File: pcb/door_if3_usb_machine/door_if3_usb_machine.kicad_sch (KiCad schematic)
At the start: 75 parts, among them J1 Conn_01x08, J2 Conn_02x05_Odd_Even, J3 Conn_01x08, Q1 IRF7343, Q2 IRF7343, Q3 IRF7343, Q4 IRF7343, Q5 IRF7343, Q6 IRF7343, U1 Pico, U2 LTV-247, U4 LTV-247

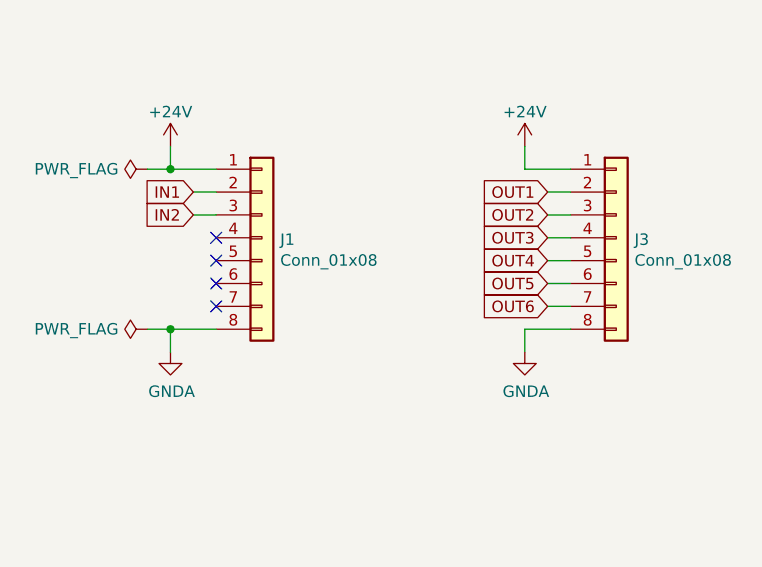
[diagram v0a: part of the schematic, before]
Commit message: completed if3_usb_machine
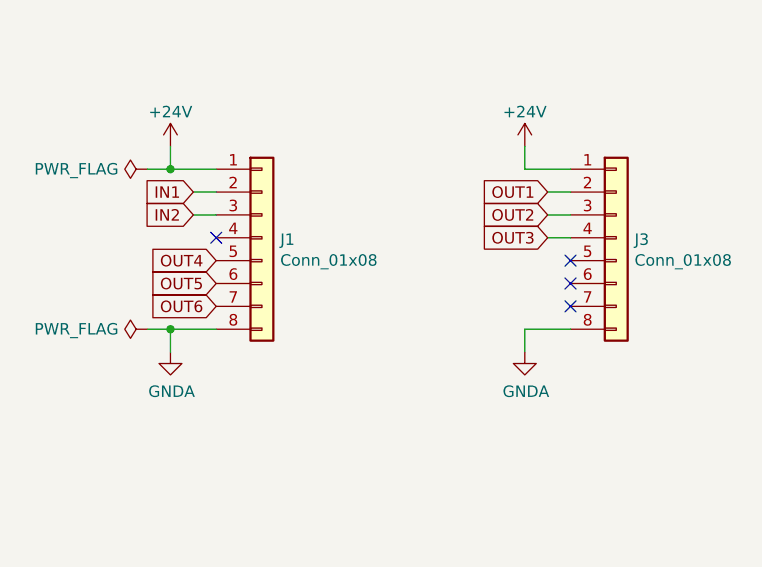
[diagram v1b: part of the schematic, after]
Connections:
- net OUT4: now also J1.5 (Pin_5); no longer J3.5 (Pin_5)
- net OUT5: now also J1.6 (Pin_6); no longer J3.6 (Pin_6)
- net OUT6: now also J1.7 (Pin_7); no longer J3.7 (Pin_7)
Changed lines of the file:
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@@
   (no_connect (at 97.79 96.52))
   (no_connect (at 113.03 68.58))
+  (no_connect (at 120.65 217.17))
+  (no_connect (at 120.65 214.63))
   (no_connect (at 113.03 55.88))
   (no_connect (at 113.03 63.5))
   (no_connect (at 113.03 50.8))
   (no_connect (at 77.47 76.2))
-  (no_connect (at 81.28 217.17))
   (no_connect (at 81.28 209.55))
-  (no_connect (at 81.28 214.63))
+  (no_connect (at 120.65 212.09))
   (no_connect (at 113.03 66.04))
-  (no_connect (at 81.28 212.09))
   (no_connect (at 77.47 78.74))
   (no_connect (at 92.71 96.52))
@@
     (stroke (width 0) (type default))
   )
-  (wire (pts (xy 118.11 217.17) (xy 120.65 217.17))
-    (stroke (width 0) (type default))
-  )
   (wire (pts (xy 271.78 154.94) (xy 274.32 154.94))
     (stroke (width 0) (type default))
@@
     (stroke (width 0) (type default))
   )
-  (wire (pts (xy 118.11 214.63) (xy 120.65 214.63))
-    (stroke (width 0) (type default))
-  )
   (wire (pts (xy 95.25 96.52) (xy 95.25 99.06))
     (stroke (width 0) (type default))
@@
   )
   (wire (pts (xy 233.68 165.1) (xy 233.68 166.37))
-    (stroke (width 0) (type default))
-  )
-  (wire (pts (xy 120.65 212.09) (xy 118.11 212.09))
     (stroke (width 0) (type default))
   )
@@
     )
   )
-  (global_label "OUT4" (shape input) (at 118.11 212.09 180)
-    (effects (font (size 1.27 1.27)) (justify right))
-    (property "Intersheetrefs" "${INTERSHEET_REFS}" (at 118.11 212.09 0)
+  (global_label "OUT4" (shape input) (at 81.28 212.09 180)
+    (effects (font (size 1.27 1.27)) (justify right))
+    (property "Intersheetrefs" "${INTERSHEET_REFS}" (at 81.28 212.09 0)
       (effects (font (size 1.27 1.27)) hide)
     )
@@
     )
   )
-  (global_label "OUT6" (shape input) (at 118.11 217.17 180)
-    (effects (font (size 1.27 1.27)) (justify right))
-    (property "Intersheetrefs" "${INTERSHEET_REFS}" (at 118.11 217.17 0)
+  (global_label "OUT6" (shape input) (at 81.28 217.17 180)
+    (effects (font (size 1.27 1.27)) (justify right))
+    (property "Intersheetrefs" "${INTERSHEET_REFS}" (at 81.28 217.17 0)
       (effects (font (size 1.27 1.27)) hide)
     )
@@
     )
   )
-  (global_label "OUT5" (shape input) (at 118.11 214.63 180)
-    (effects (font (size 1.27 1.27)) (justify right))
-    (property "Intersheetrefs" "${INTERSHEET_REFS}" (at 118.11 214.63 0)
-      (effects (font (size 1.27 1.27)) hide)
-    )
+  (global_label "OUT5" (shape input) (at 81.28 214.63 180)
+    (effects (font (size 1.27 1.27)) (justify right))
+    (property "Intersheetrefs" "${INTERSHEET_REFS}" (at 81.28 214.63 0)
+      (effects (font (size 1.27 1.27)) hide)
+    )
